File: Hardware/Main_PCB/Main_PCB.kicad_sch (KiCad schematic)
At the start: 29 parts, among them J101 Conn_01x08_Pin, J102 Conn_01x03_Pin, U1 ICM-42688-P, U101 NRF24L01_Breakout, U2 TPS62170DSG, U3 TPS61175PWPR

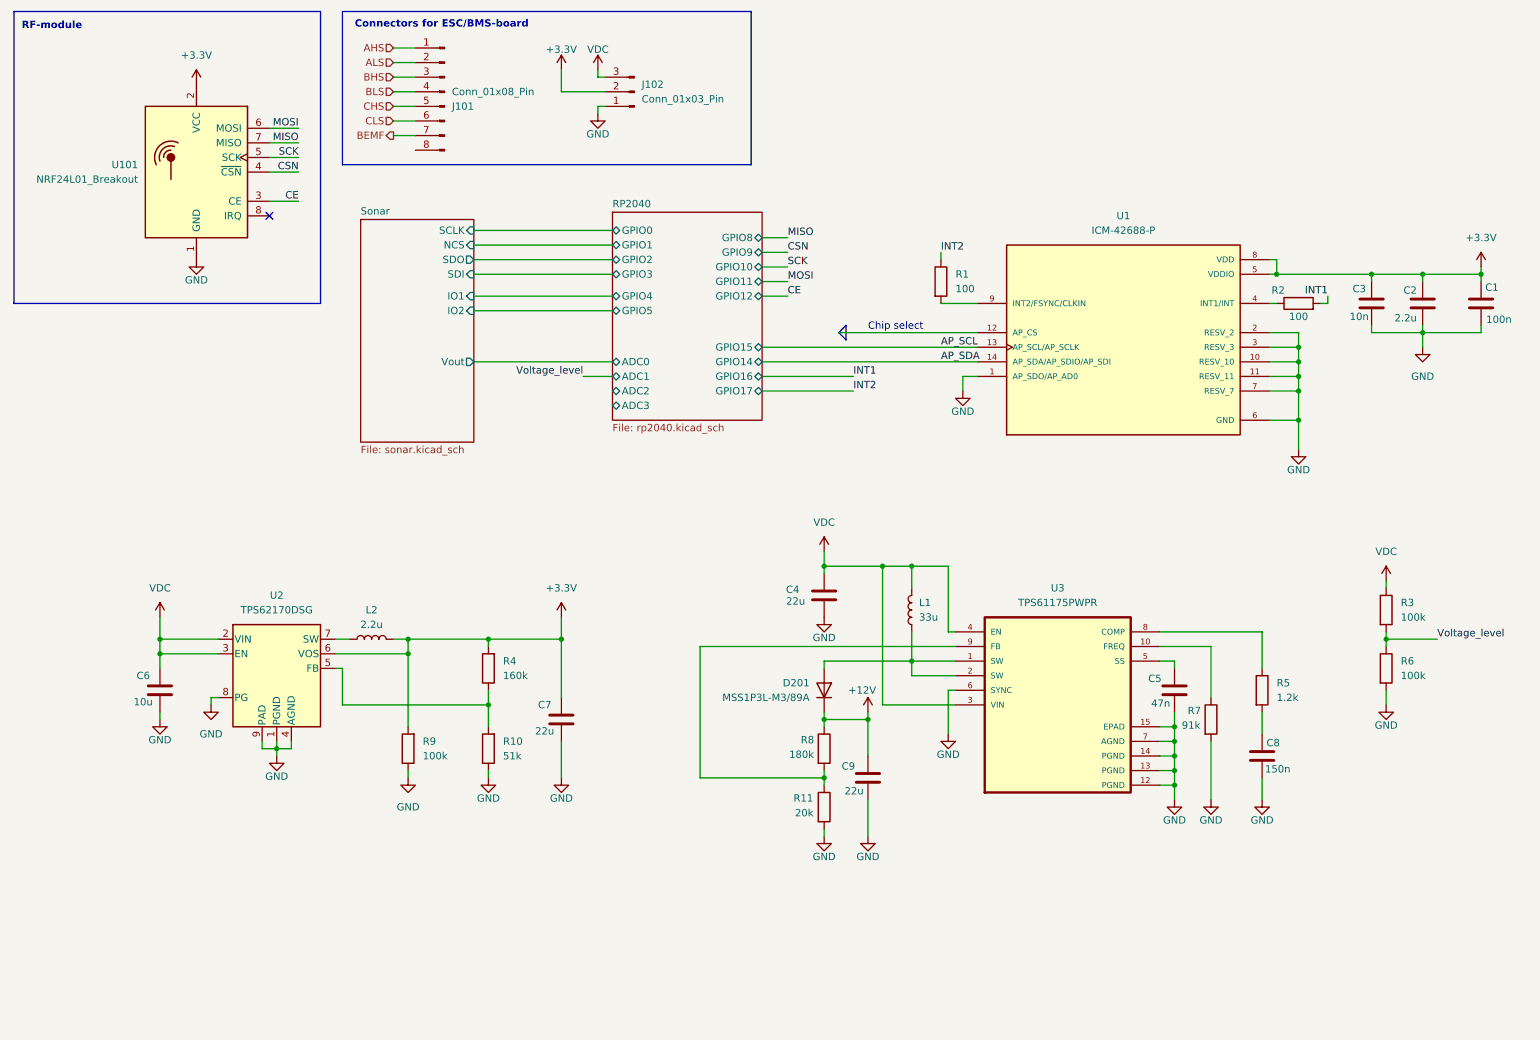
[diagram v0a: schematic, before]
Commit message: Modifications to the MainPCB
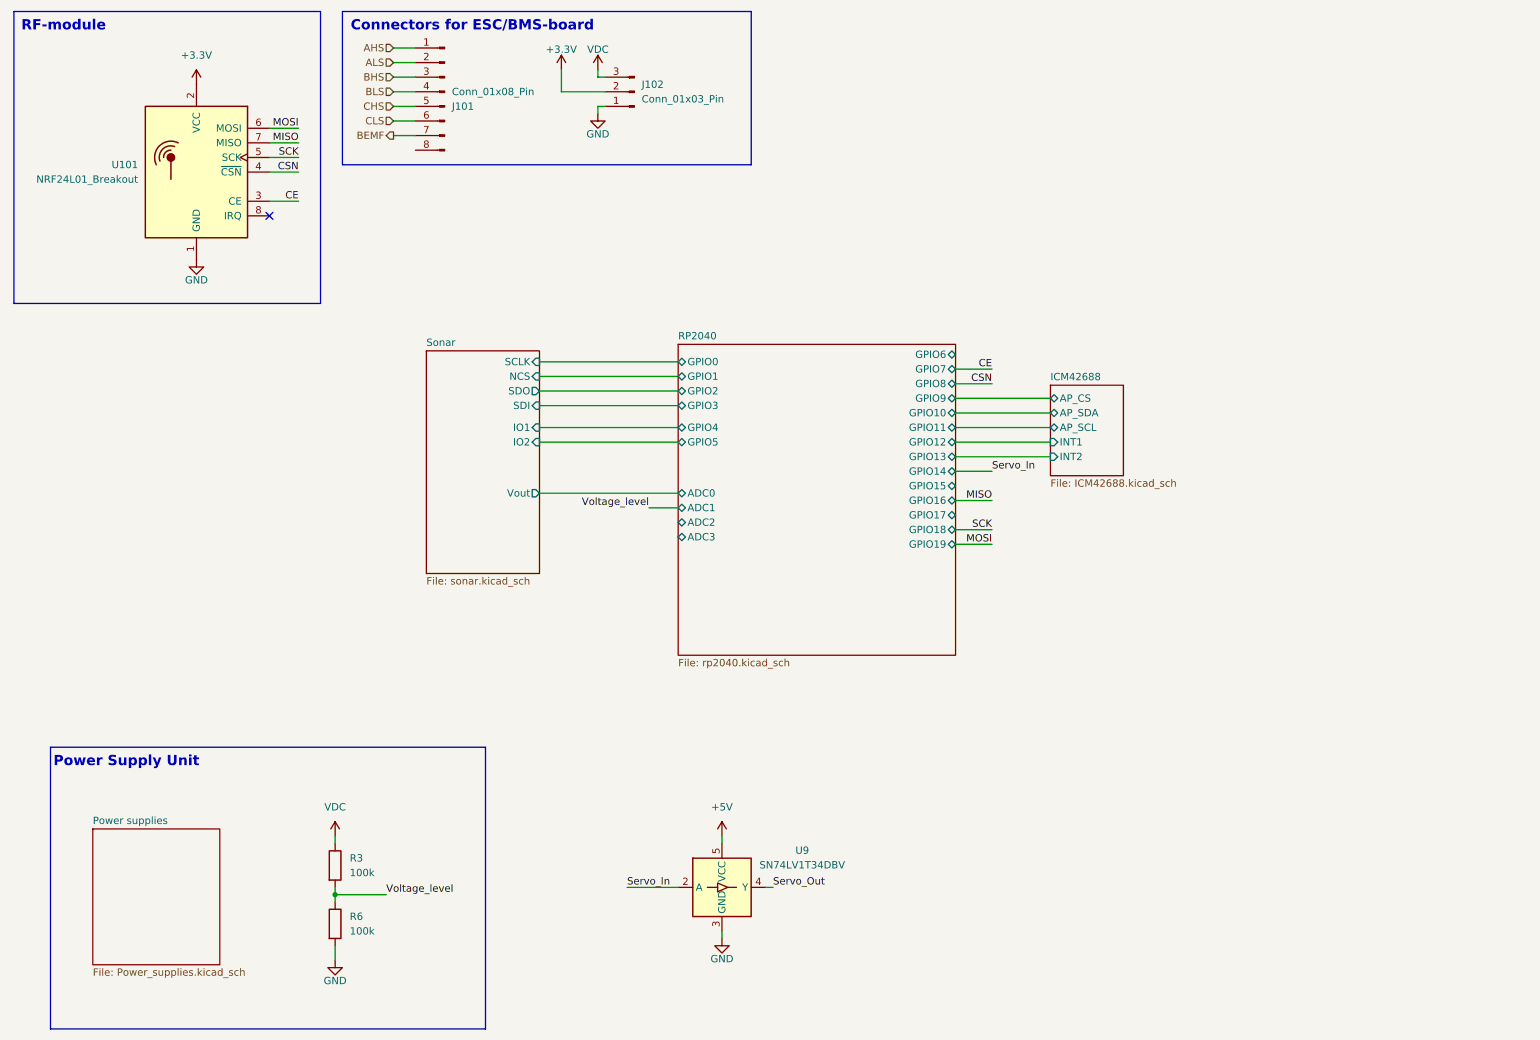
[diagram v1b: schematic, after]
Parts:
- removed C1: 100n, Capacitor_SMD:C_0805_2012Metric_Pad1.18x1.45mm_HandSolder, symbol Device:C
- removed C2: 2.2u, Capacitor_SMD:C_0805_2012Metric_Pad1.18x1.45mm_HandSolder, symbol Device:C
- removed C3: 10n, Capacitor_SMD:C_0805_2012Metric_Pad1.18x1.45mm_HandSolder, symbol Device:C
- removed C4, C7, C9: 22u, Capacitor_SMD:C_0805_2012Metric_Pad1.18x1.45mm_HandSolder, symbol Device:C
- removed C5: 47n, Capacitor_SMD:C_0805_2012Metric_Pad1.18x1.45mm_HandSolder, symbol Device:C
- removed C6: 10u, Capacitor_SMD:C_0805_2012Metric_Pad1.18x1.45mm_HandSolder, symbol Device:C
- removed C8: 150n, Capacitor_SMD:C_0805_2012Metric_Pad1.18x1.45mm_HandSolder, symbol Device:C
- removed D201: MSS1P3L-M3/89A, Diode_SMD:Vishay_SMPA, symbol Diode:S2JTR
- removed L1: 33u, MainPCB:IND_SRR6038-100Y, symbol Device:L
- removed L2: 2.2u, Inductor_SMD:L_APV_ANR252012, symbol Device:L
- removed R1, R2: 100, Resistor_SMD:R_0603_1608Metric_Pad0.98x0.95mm_HandSolder, symbol Device:R
- removed R10: 51k, Resistor_SMD:R_0603_1608Metric_Pad0.98x0.95mm_HandSolder, symbol Device:R
- removed R11: 20k, Resistor_SMD:R_0603_1608Metric_Pad0.98x0.95mm_HandSolder, symbol Device:R
- removed R4: 160k, Resistor_SMD:R_0603_1608Metric_Pad0.98x0.95mm_HandSolder, symbol Device:R
- removed R5: 1.2k, Resistor_SMD:R_0603_1608Metric_Pad0.98x0.95mm_HandSolder, symbol Device:R
- removed R7: 91k, Resistor_SMD:R_0603_1608Metric_Pad0.98x0.95mm_HandSolder, symbol Device:R
- removed R8: 180k, Resistor_SMD:R_0603_1608Metric_Pad0.98x0.95mm_HandSolder, symbol Device:R
- removed R9: 100k, Resistor_SMD:R_0603_1608Metric_Pad0.98x0.95mm_HandSolder, symbol Device:R
- removed U1: ICM-42688-P, ICM-42688-P:PQFN50P300X250X97-14N, symbol ICM-42688-P:ICM-42688-P
- removed U2: TPS62170DSG, Package_SON:WSON-8-1EP_2x2mm_P0.5mm_EP0.9x1.6mm_ThermalVias, symbol Regulator_Switching:TPS62170DSG
- removed U3: TPS61175PWPR, TPS61175PWPR:IC_TPS27S100BPWPR, symbol TPS61175PWPR:TPS61175PWPR
- added U9: SN74LV1T34DBV, Package_TO_SOT_SMD:SOT-23-5, symbol Logic_LevelTranslator:SN74LV1T34DBV
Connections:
- net GND: now also U9.3 (GND)
- new net +5V: U9.5 (VCC)
- new net Servo_In: U9.2 (A)
- new net Servo_Out: U9.4 (Y)
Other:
- added sheet ICM42688 (ICM42688.kicad_sch)
- added sheet Power supplies (Power_supplies.kicad_sch)
- sheet RP2040 ports: added GPIO13, GPIO18, GPIO19, GPIO6, GPIO7; removed none
- note added: "Power Supply Unit"
- note removed: "Chip select"
- moved on the sheet: R3, R6
